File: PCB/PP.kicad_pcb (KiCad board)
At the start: 2 copper layers, 96.5 x 58.4 mm, 39 parts, among them Q1 Q_PMOS_DGS, Q2 Q_NMOS_DGS, Q3 Q_PMOS_DGS, Q4 Q_NMOS_DGS, U1 ESP32_DEVKITV1

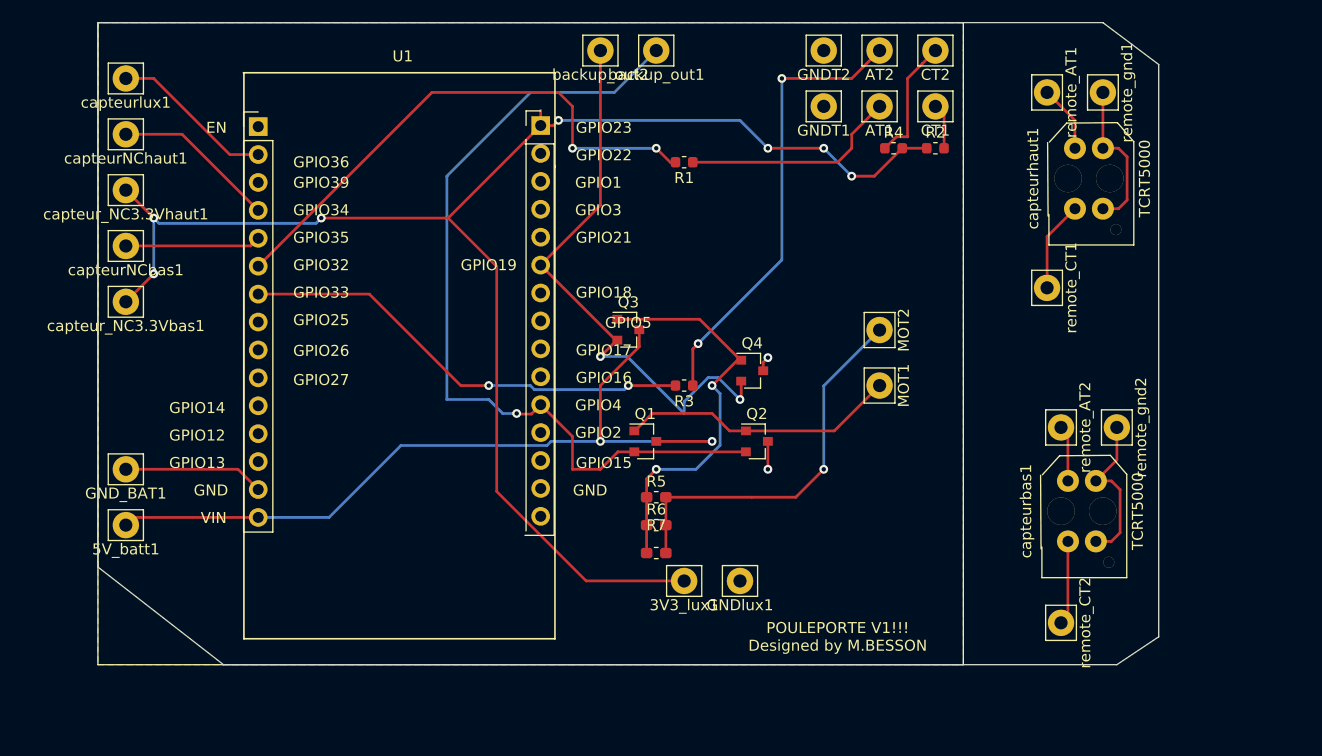
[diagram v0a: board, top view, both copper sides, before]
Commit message: Update pouleporte releaseV2
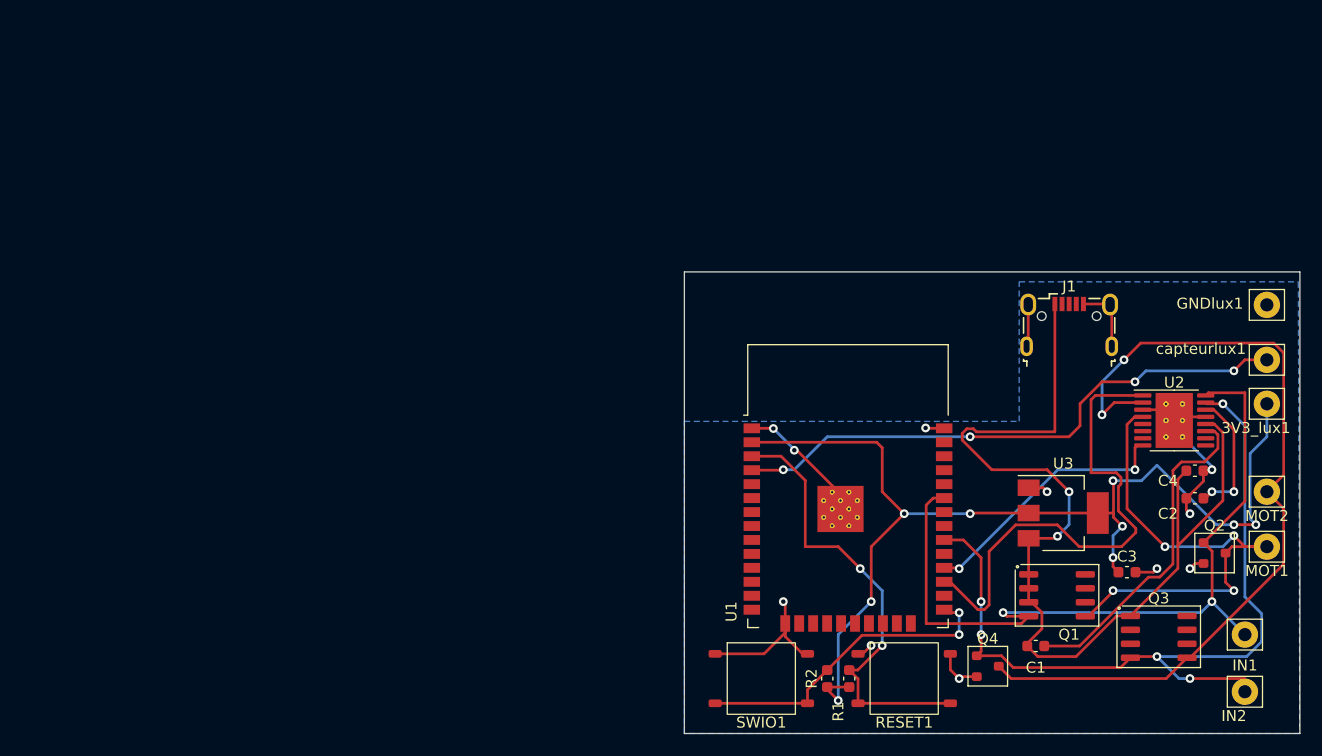
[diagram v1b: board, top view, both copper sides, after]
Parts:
- removed 5V_batt1, AT1, AT2, CT1, CT2, GNDT1, GNDT2, GND_BAT1, backup_out1, backup_out2, capteurNCbas1, capteurNChaut1, capteur_NC3.3Vbas1, capteur_NC3.3Vhaut1, remote_AT1, remote_AT2, remote_CT1, remote_CT2, remote_gnd1, remote_gnd2: Conn_01x01, Connector_Pin:Pin_D1.2mm_L11.3mm_W3.0mm_Flat
- removed R3: 33, Resistor_SMD:R_0603_1608Metric
- removed R4: 10k, Resistor_SMD:R_0603_1608Metric
- removed R5, R6, R7: 12, Resistor_SMD:R_0603_1608Metric_Pad1.05x0.95mm_HandSolder
- removed capteurbas1, capteurhaut1: TCRT5000, wemos:TCRT5000
- added C1: 0.01uF, Capacitor_SMD:C_0603_1608Metric, F.Cu at (126.0, 77.0)
- added C2: 2.2uf, Capacitor_SMD:C_0603_1608Metric, F.Cu at (140.4, 63.6)
- added C3: 4.7uF, Capacitor_SMD:C_0603_1608Metric, F.Cu at (134.3, 70.3)
- added C4: 1uF, Capacitor_SMD:C_0603_1608Metric, F.Cu at (140.4, 61.1)
- added IN1: Conn_01x01, Connector_Pin:Pin_D1.2mm_L11.3mm_W3.0mm_Flat, F.Cu at (145.0, 76.0)
- added IN2: Conn_01x01, Connector_Pin:Pin_D1.2mm_L11.3mm_W3.0mm_Flat, F.Cu at (145.0, 81.2)
- added J1: USB_B_Micro, Connector_USB:USB_Micro-B_Wuerth_629105150521, F.Cu at (129.0, 47.8)
- added RESET1: SW_Push_Open, Library:interrupteur, F.Cu at (109.8, 77.8)
- added SWIO1: SW_Push_Open, Library:interrupteur, F.Cu at (96.8, 77.8)
- added U2: DRV8833PWP, Package_SO:HTSSOP-16-1EP_4.4x5mm_P0.65mm_EP3.4x5mm_Mask2.46x2.31mm_ThermalVias, F.Cu at (138.6, 56.5)
- added U3: AP7361C-33E, Package_TO_SOT_SMD:SOT-223-3_TabPin2, F.Cu at (128.5, 64.9)
- Q1, Q3: value Q_PMOS_DGS -> AO4425; footprint Package_TO_SOT_SMD:SOT-23 -> Package_SO_AKL:SO-8_3.9x4.9mm_P1.27mm
- Q2, Q4: value Q_NMOS_DGS -> AO3406; footprint Package_TO_SOT_SMD:SOT-23 -> Package_TO_SOT_SMD_AKL:SOT-23
- R1: value 33 -> 10k; footprint Resistor_SMD:R_0603_1608Metric -> Capacitor_SMD:C_0603_1608Metric
- R2: footprint Resistor_SMD:R_0603_1608Metric -> Capacitor_SMD:C_0603_1608Metric
- U1: value ESP32_DEVKITV1 -> ESP32-WROOM-32; footprint wemos:devkt1_online -> RF_Module:ESP32-WROOM-32
- moved capteurlux1 106.9 mm to (147.0, 51.0)
- moved U1 56.0 mm to (108.9, 65.5)
- moved Q3 55.8 mm to (137.2, 76.2)
- moved 3V3_lux1 55.4 mm to (147.0, 55.0)
- moved GNDlux1 54.1 mm to (147.0, 46.0)
- moved R1 49.3 mm to (109.0, 80.0), turned to 90 degrees
- moved R2 49.2 mm to (107.0, 80.0), turned to 90 degrees
- moved Q2 42.9 mm to (142.2, 68.6)
- moved Q1 40.0 mm to (127.9, 72.4)
- moved MOT2 38.2 mm to (147.0, 63.0), turned to 0 degrees
- moved MOT1 38.2 mm to (147.0, 68.0), turned to 0 degrees
- moved Q4 34.4 mm to (121.6, 78.9)
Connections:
- Q1 pad 1: Net-(MOT1-Pad1) -> 5V
- Q1 pad 2: Net-(Q1-Pad2) -> 5V
- Q2 pad 1: Net-(MOT1-Pad1) -> Net-(backup_out1-Pad1)
- Q2 pad 2: Net-(Q1-Pad2) -> GND
- Q2 pad 3: GND -> Net-(MOT1-Pad1)
- Q3 pad 1: Net-(Q3-Pad1) -> 5V
- Q3 pad 2: Net-(Q3-Pad2) -> unconnected-(Q3-Pad2)
- Q3 pad 3: 5V -> unconnected-(Q3-Pad3)
- Q4 pad 1: Net-(Q3-Pad1) -> Net-(backup_out2-Pad1)
- Q4 pad 2: Net-(Q3-Pad2) -> GND
- Q4 pad 3: GND -> Net-(MOT2-Pad1)
- R1 pad 1: Net-(AT1-Pad1) -> VCC
- R2 pad 2: Net-(CT1-Pad1) -> Net-(R2-Pad2)
- U1 pad 1: Net-(U1-Pad1) -> GND
- U1 pad 10: Net-(U1-Pad10) -> unconnected-(U1-Pad10)
- U1 pad 11: Net-(U1-Pad11) -> unconnected-(U1-Pad11)
- U1 pad 12: Net-(U1-Pad12) -> unconnected-(U1-Pad12)
- U1 pad 13: Net-(U1-Pad13) -> unconnected-(U1-Pad13)
- U1 pad 14: GND -> unconnected-(U1-Pad14)
- U1 pad 15: 5V -> GND
- U1 pad 16: Net-(U1-Pad16) -> unconnected-(U1-Pad16)
- U1 pad 17: Net-(U1-Pad17) -> unconnected-(U1-Pad17)
- U1 pad 18: Net-(U1-Pad18) -> unconnected-(U1-Pad18)
- U1 pad 19: Net-(U1-Pad19) -> unconnected-(U1-Pad19)
- U1 pad 2: Net-(U1-Pad2) -> VCC
- U1 pad 20: Net-(Q1-Pad2) -> unconnected-(U1-Pad20)
- U1 pad 21: Net-(U1-Pad21) -> unconnected-(U1-Pad21)
- U1 pad 22: Net-(U1-Pad22) -> unconnected-(U1-Pad22)
- U1 pad 23: Net-(U1-Pad23) -> unconnected-(U1-Pad23)
- U1 pad 24: Net-(U1-Pad24) -> unconnected-(U1-Pad24)
- U1 pad 25: Net-(Q3-Pad2) -> Net-(R2-Pad2)
- U1 pad 26: Net-(U1-Pad26) -> unconnected-(U1-Pad26)
- U1 pad 29: Net-(U1-Pad29) -> unconnected-(U1-Pad29)
- U1 pad 3: Net-(U1-Pad3) -> Net-(R1-Pad2)
- U1 pad 30: VCC -> Net-(backup_out2-Pad1)
- U1 pad 4: Net-(U1-Pad4) -> Net-(capteurlux1-Pad1)
- U1 pad 5: Net-(U1-Pad5) -> unconnected-(U1-Pad5)
- U1 pad 6: Net-(R1-Pad2) -> unconnected-(U1-Pad6)
- U1 pad 7: Net-(R3-Pad2) -> unconnected-(U1-Pad7)
- U1 pad 8: Net-(U1-Pad8) -> unconnected-(U1-Pad8)
- U1 pad 9: Net-(U1-Pad9) -> unconnected-(U1-Pad9)
- capteurlux1 pad 1: Net-(U1-Pad2) -> Net-(capteurlux1-Pad1)
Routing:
- net Net-(Q1-Pad2): track 77.1 -> 0.00 mm, vias 1 -> 0
- net Net-(backup_out2-Pad1): track 0.00 -> 74.0 mm, vias 0 -> 5
- net Net-(backup_out1-Pad1): track 0.00 -> 73.0 mm, vias 0 -> 2
- net Net-(Q3-Pad2): track 53.1 -> 0.00 mm, vias 2 -> 0
- net Net-(capteurlux1-Pad1): track 0.00 -> 52.2 mm, vias 0 -> 4
- net GND: track 16.7 -> 65.7 mm, vias 2 -> 11
- net Net-(U1-Pad27): track 0.00 -> 46.1 mm
- net Net-(R3-Pad2): track 41.7 -> 0.00 mm, vias 2 -> 0
- net Net-(MOT2-Pad1): track 35.3 -> 76.7 mm, vias 1 -> 2
- net Net-(AT2-Pad1): track 41.2 -> 0.00 mm, vias 2 -> 0
- net VCC: track 138.4 -> 98.0 mm, vias 7 -> 9
- net Net-(Q3-Pad1): track 36.8 -> 0.00 mm, vias 2 -> 0
- net Net-(C1-Pad2): track 0.00 -> 30.7 mm
- net Net-(R2-Pad2): track 0.00 -> 29.0 mm, vias 0 -> 2
- net Net-(U1-Pad28): track 0.00 -> 23.9 mm, vias 0 -> 2
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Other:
- board size 96.5 x 58.4 mm -> 56 x 42 mm
- net class Default removed
- board text added: "Pouleporte V2 Designed by MBE"
- board text removed: "POULEPORTE V1!!! Designed by M.BESSON"
